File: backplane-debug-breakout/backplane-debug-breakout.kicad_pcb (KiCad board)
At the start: 2 copper layers, 65 x 50.5 mm, 11 parts, among them J1 Conn_02x08_Odd_Even, J2 Conn_01x04, J3 Conn_01x01_Socket, J4 Conn_01x01_Socket, J5 Conn_01x04, SW1 SW_Push, SW2 SW_DPST_x2, U1 UMFT234XF

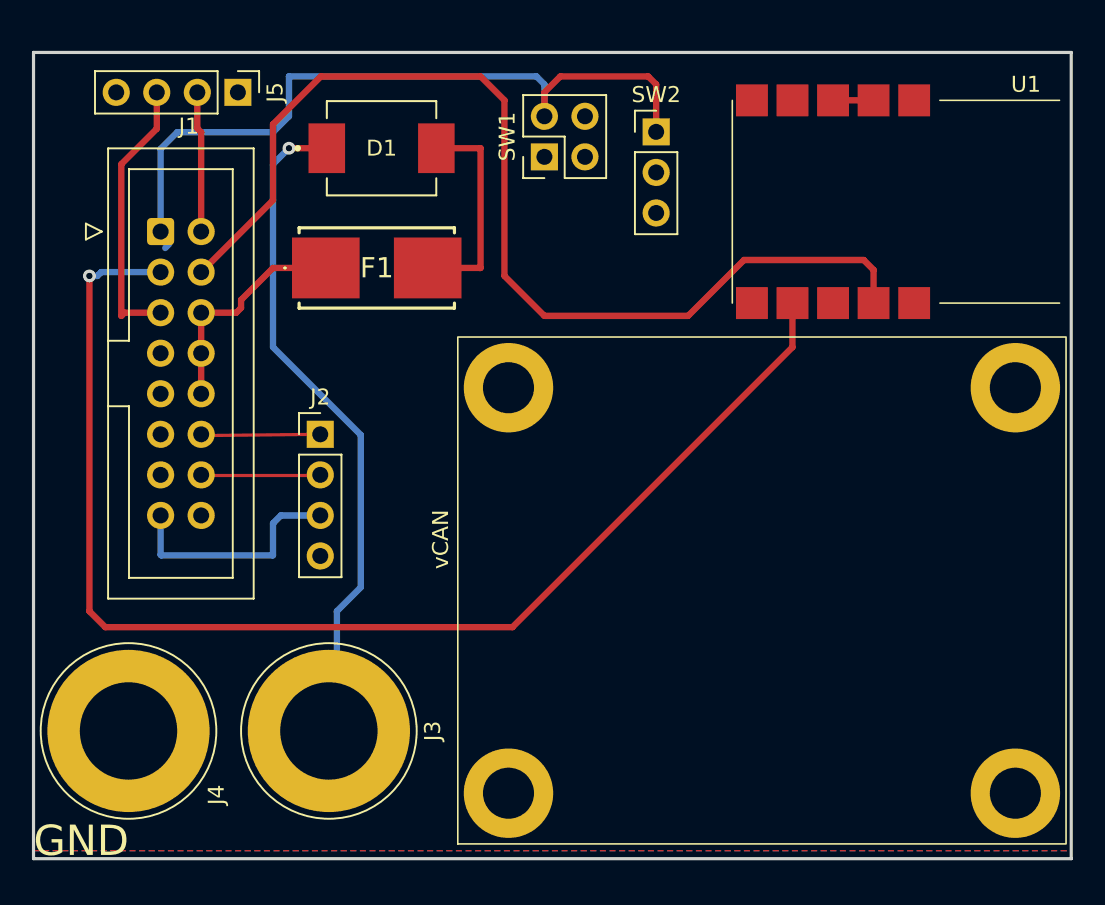
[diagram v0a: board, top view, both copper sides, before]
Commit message: modified pcb
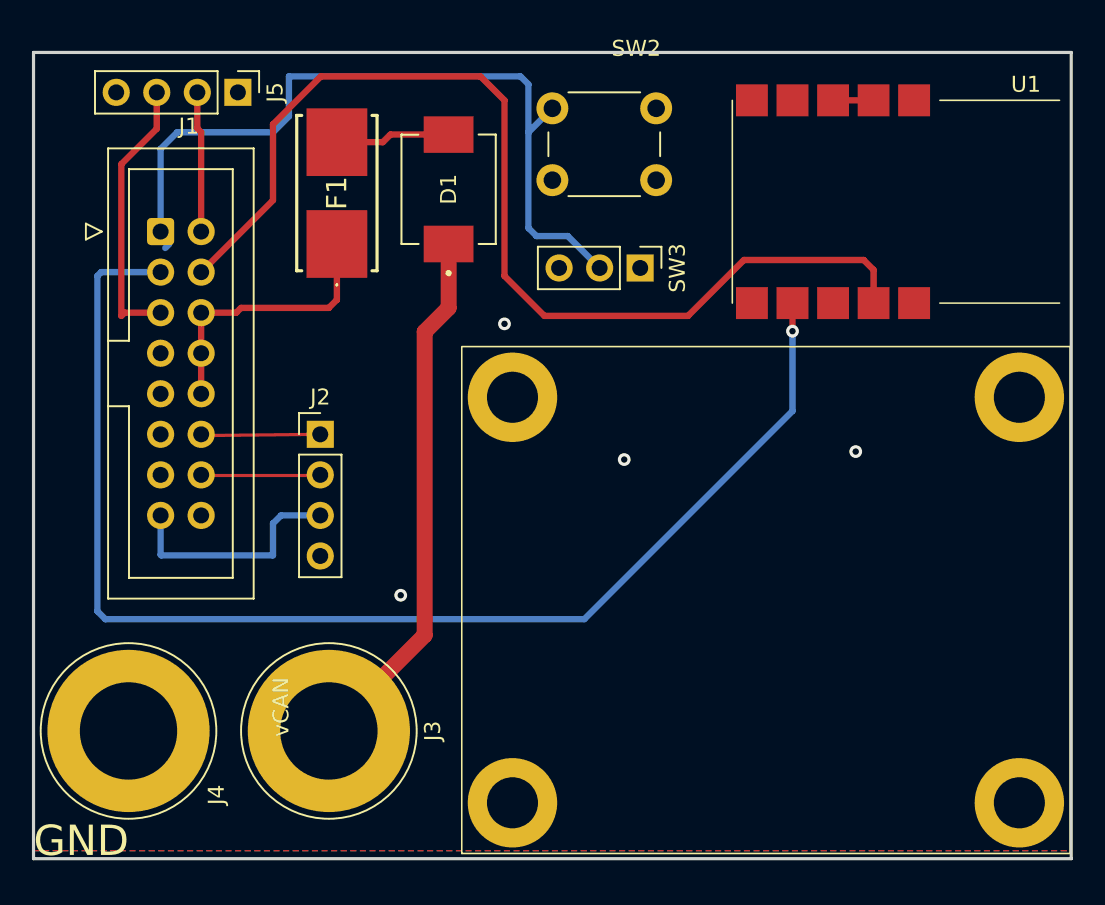
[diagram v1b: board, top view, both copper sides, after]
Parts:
- removed SW1: SW_Push, Connector_PinHeader_2.54mm:PinHeader_2x02_P2.54mm_Vertical
- added SW3: EG1218, Connector_PinHeader_2.54mm:PinHeader_1x03_P2.54mm_Vertical, F.Cu at (135.0, 72.5)
- SW2: value SW_DPST_x2 -> SW_Omron_B3FS; footprint Connector_PinHeader_2.54mm:PinHeader_1x03_P2.54mm_Vertical -> Button_Switch_THT:SW_PUSH_6mm
- moved F1 5.31 mm to (116.0, 67.8), turned to 90 degrees
- moved D1 4.92 mm to (123.0, 67.6), turned to 90 degrees
- moved SW2 3.02 mm to (136.0, 67.0), turned to 180 degrees
- moved vCAN 0.65 mm to (127.0, 106.0)
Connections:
- net Net-(J1-Pin_10) renamed /VBUS
- SW2 pad 1: /SD -> GND
- SW2 pad 2: GND -> /SD
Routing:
- net Net-(D1-A): track 42.4 -> 34.3 mm, vias 1 -> 0
- net Net-(D1-K): track 13.4 -> 7.20 mm
- net /VBUS: track 14.3 -> 17.4 mm
- net /SD: track 47.1 -> 48.7 mm
- net /C3-UART-TX: track 80.0 -> 81.0 mm
- net GND: vias 0 -> 4
